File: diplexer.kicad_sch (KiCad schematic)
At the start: 27 parts, among them J1 Conn_Coaxial, J2 Conn_Coaxial, J3 Conn_Coaxial, J4 Conn_01x01_Pin, J5 Conn_01x01_Pin, J6 Conn_01x01_Pin, J7 Conn_01x01_Pin

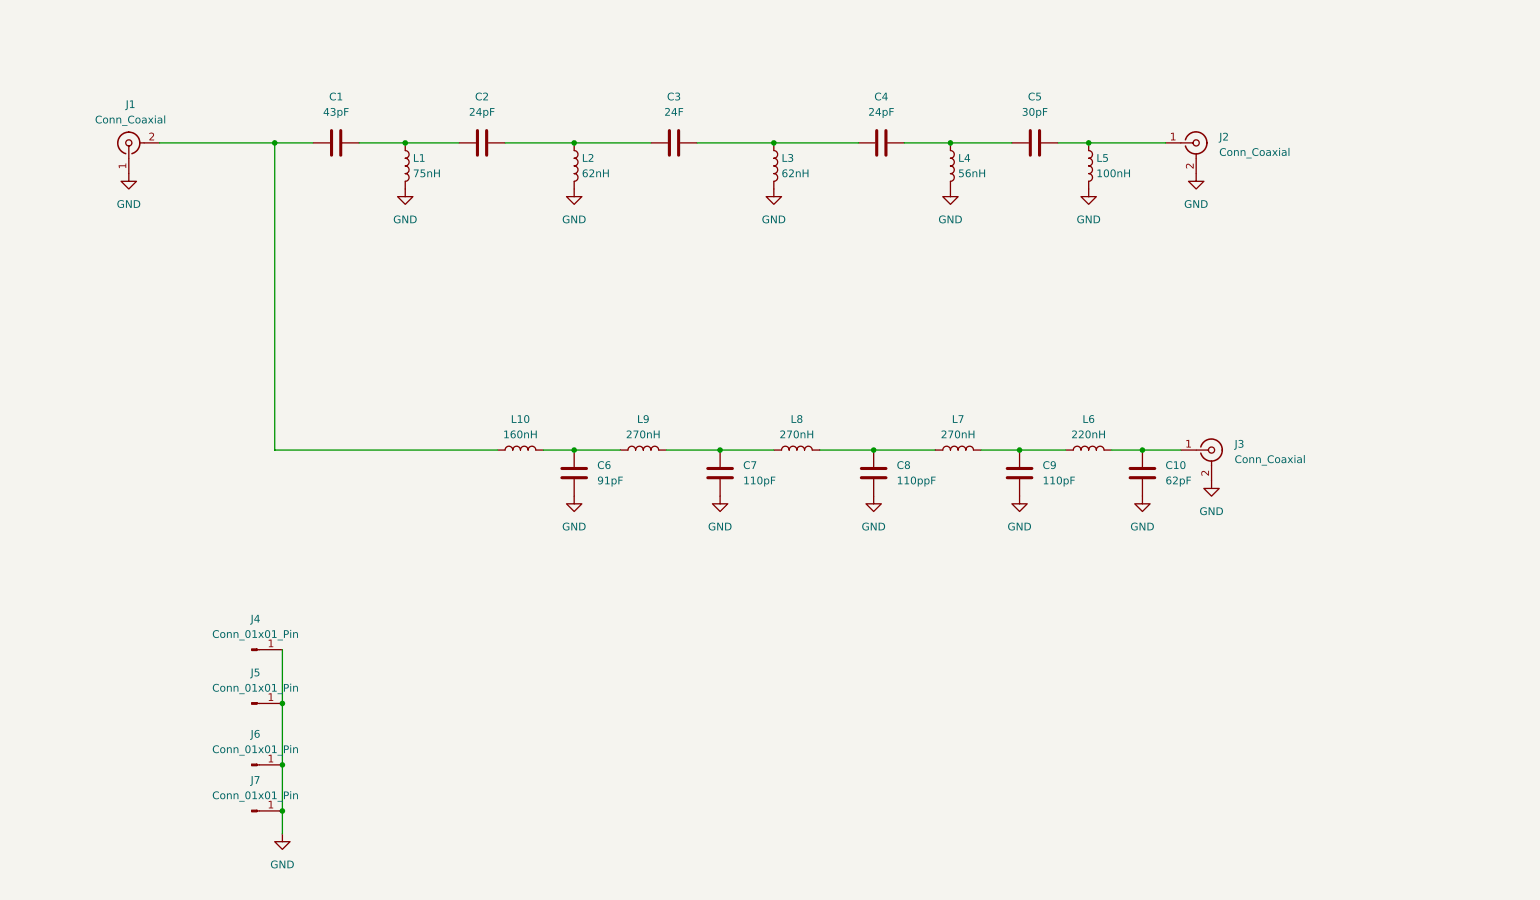
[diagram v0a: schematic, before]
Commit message: Add files via upload
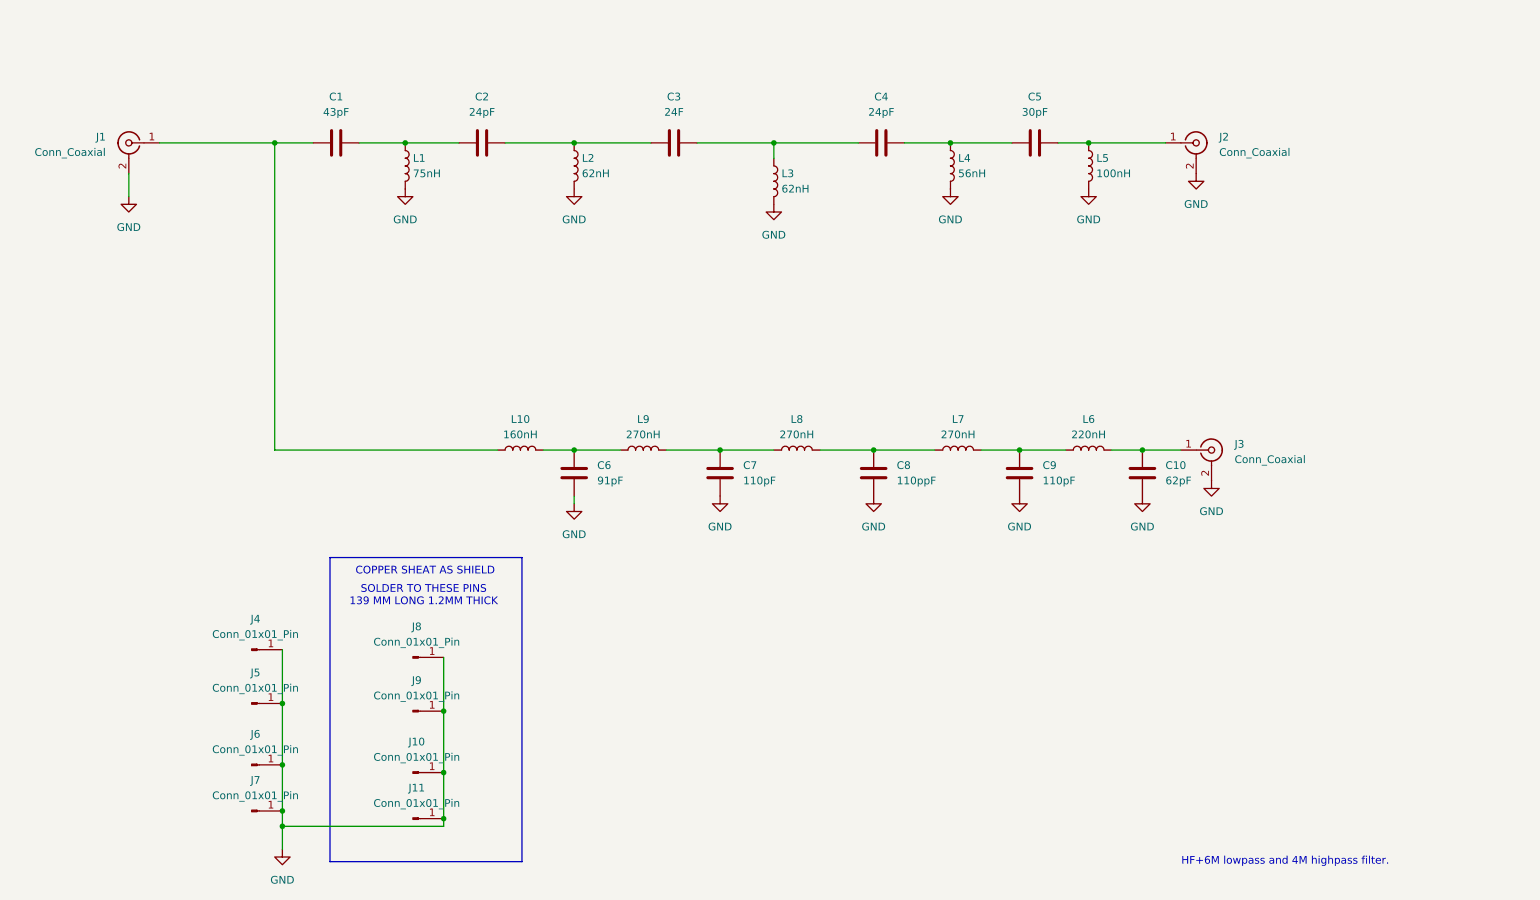
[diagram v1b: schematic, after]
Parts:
- added J10, J11, J8, J9: Conn_01x01_Pin, MountingHole:MountingHole_3.2mm_M3_DIN965_Pad, symbol Connector:Conn_01x01_Pin
- J4, J5, J6, J7: footprint MountingHole:MountingHole_3.2mm_M3 -> MountingHole:MountingHole_3.2mm_M3_DIN965_Pad
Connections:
- net GND: now also J1.2 (Ext), J10.1 (Pin_1), J11.1 (Pin_1), J8.1 (Pin_1), J9.1 (Pin_1); no longer J1.1 (In)
- net at C1.1, L10.1: now also J1.1 (In); no longer J1.2 (Ext)
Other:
- note added: "COPPER SHEAT AS SHIELD"
- note added: "HF+6M lowpass and 4M highpass filter."
- note added: "SOLDER TO THESE PINS 139 MM LONG 1.2MM THICK"
- moved on the sheet: J1, L3

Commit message: Add files via upload
Updated capacitors foot prints to 2525 (QEEV Series)
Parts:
- C1, C10, C2, C3, C4, C5, C6, C7, C8, C9: footprint Capacitor_SMD:C_2220_5750Metric -> sparkfun-electromech:2525
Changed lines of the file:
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@@
 			)
 		)
-		(property "Footprint" "Capacitor_SMD:C_2220_5750Metric"
+		(property "Footprint" "sparkfun-electromech:2525"
 			(at 105.7148 104.14 0)
 			(effects
@@
 			)
 		)
-		(property "Footprint" "Capacitor_SMD:C_2220_5750Metric"
+		(property "Footprint" "sparkfun-electromech:2525"
 			(at 186.69 52.3748 0)
 			(effects
@@
 			)
 		)
-		(property "Footprint" "Capacitor_SMD:C_2220_5750Metric"
+		(property "Footprint" "sparkfun-electromech:2525"
 			(at 161.29 52.3748 0)
 			(effects
@@
 			)
 		)
-		(property "Footprint" "Capacitor_SMD:C_2220_5750Metric"
+		(property "Footprint" "sparkfun-electromech:2525"
 			(at 179.3748 104.14 0)
 			(effects
@@
 			)
 		)
-		(property "Footprint" "Capacitor_SMD:C_2220_5750Metric"
+		(property "Footprint" "sparkfun-electromech:2525"
 			(at 95.25 52.3748 0)
 			(effects
@@
 			)
 		)
-		(property "Footprint" "Capacitor_SMD:C_2220_5750Metric"
+		(property "Footprint" "sparkfun-electromech:2525"
 			(at 199.6948 104.14 0)
 			(effects
@@
 			)
 		)
-		(property "Footprint" "Capacitor_SMD:C_2220_5750Metric"
+		(property "Footprint" "sparkfun-electromech:2525"
 			(at 129.8448 104.14 0)
 			(effects
@@
 			)
 		)
-		(property "Footprint" "Capacitor_SMD:C_2220_5750Metric"
+		(property "Footprint" "sparkfun-electromech:2525"
 			(at 71.12 52.3748 0)
 			(effects
@@
 			)
 		)
-		(property "Footprint" "Capacitor_SMD:C_2220_5750Metric"
+		(property "Footprint" "sparkfun-electromech:2525"
 			(at 155.2448 104.14 0)
 			(effects
@@
 			)
 		)
-		(property "Footprint" "Capacitor_SMD:C_2220_5750Metric"
+		(property "Footprint" "sparkfun-electromech:2525"
 			(at 127 52.3748 0)
 			(effects

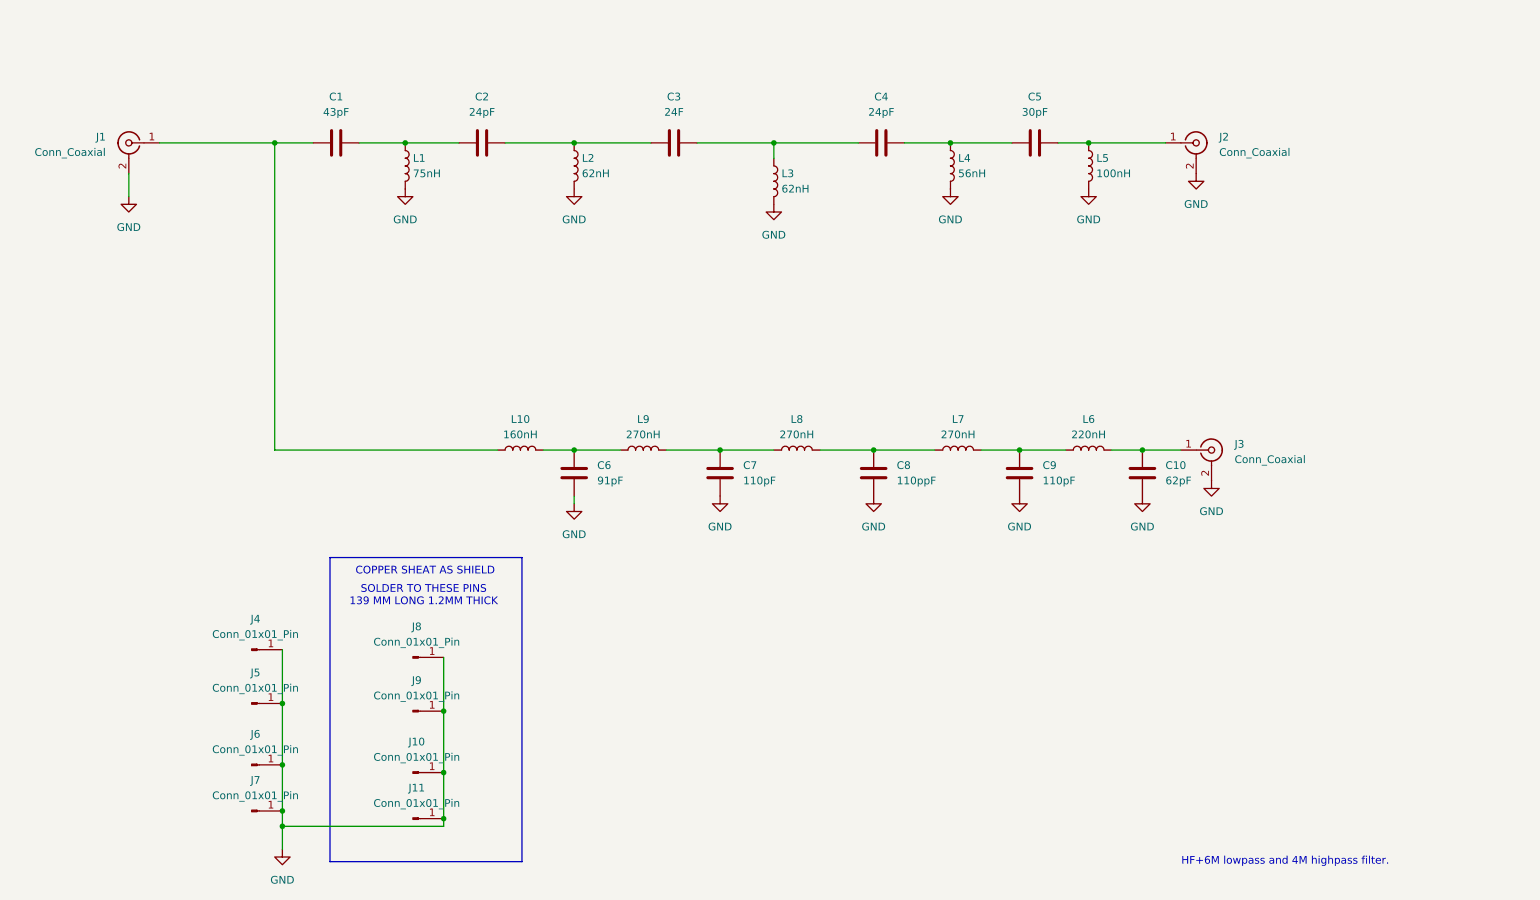
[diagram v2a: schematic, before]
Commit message: Add files via upload
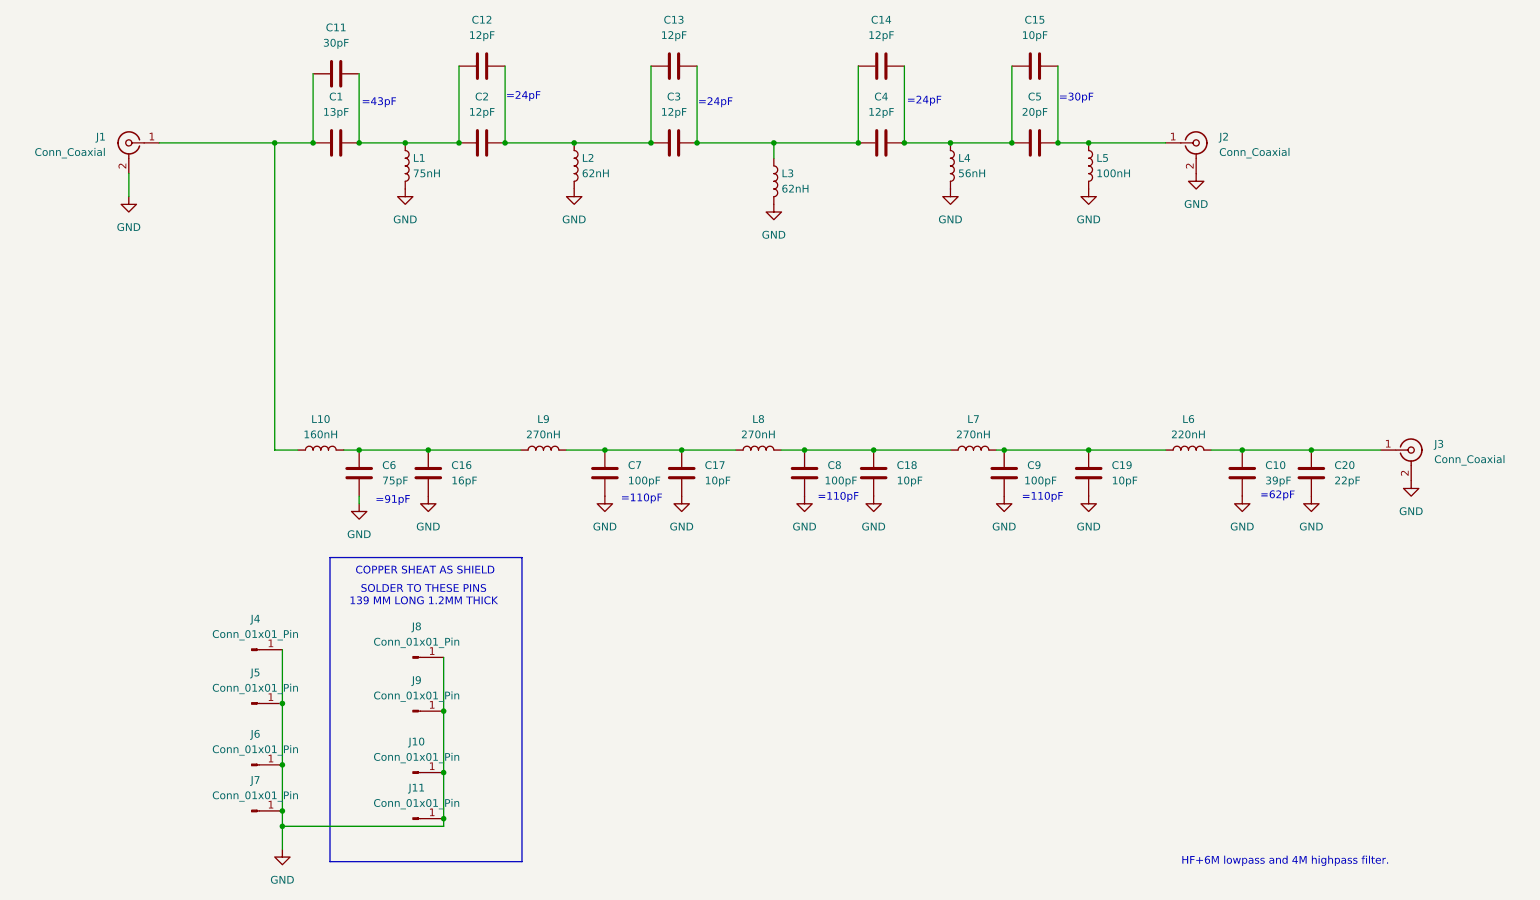
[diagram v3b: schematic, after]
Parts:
- added C11: 30pF, sparkfun-electromech:1111, symbol Device:C
- added C12, C13, C14: 12pF, sparkfun-electromech:1111, symbol Device:C
- added C15, C17, C18, C19: 10pF, sparkfun-electromech:1111, symbol Device:C
- added C16: 16pF, sparkfun-electromech:1111, symbol Device:C
- added C20: 22pF, sparkfun-electromech:1111, symbol Device:C
- C1: value 43pF -> 13pF; footprint sparkfun-electromech:2525 -> sparkfun-electromech:1111
- C10: value 62pF -> 39pF; footprint sparkfun-electromech:2525 -> sparkfun-electromech:1111
- C2, C4: value 24pF -> 12pF; footprint sparkfun-electromech:2525 -> sparkfun-electromech:1111
- C3: value 24F -> 12pF; footprint sparkfun-electromech:2525 -> sparkfun-electromech:1111
- C5: value 30pF -> 20pF; footprint sparkfun-electromech:2525 -> sparkfun-electromech:1111
- C6: value 91pF -> 75pF; footprint sparkfun-electromech:2525 -> sparkfun-electromech:1111
- C7, C9: value 110pF -> 100pF; footprint sparkfun-electromech:2525 -> sparkfun-electromech:1111
- C8: value 110ppF -> 100pF; footprint sparkfun-electromech:2525 -> sparkfun-electromech:1111
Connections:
- net GND: now also C16.2, C17.2, C18.2, C19.2, C20.2
- net at C6.2, L10.2, L9.1: now also C16.1
- net at C4.2, C5.1, L4.1: now also C14.2, C15.1
- net at C5.2, J2.1 (In), L5.1: now also C15.2
- net at C3.2, C4.1, L3.1: now also C13.2, C14.1
- net at C1.1, J1.1 (In), L10.1: now also C11.1
- net at C7.2, L8.1, L9.2: now also C17.1
- net at C8.2, L7.1, L8.2: now also C18.1
- net at C9.2, L6.1, L7.2: now also C19.1
- net at C1.2, C2.1, L1.1: now also C11.2, C12.1
- net at C2.2, C3.1, L2.1: now also C12.2, C13.1
- net at C10.2, J3.1 (In), L6.2: now also C20.1
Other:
- note added: "=110pF"
- note added: "=24pF"
- note added: "=30pF"
- note added: "=43pF"
- note added: "=62pF"
- note added: "=91pF"
- moved on the sheet: C10, C6, C7, C8, C9, J3, L10, L6, L7, L8, L9

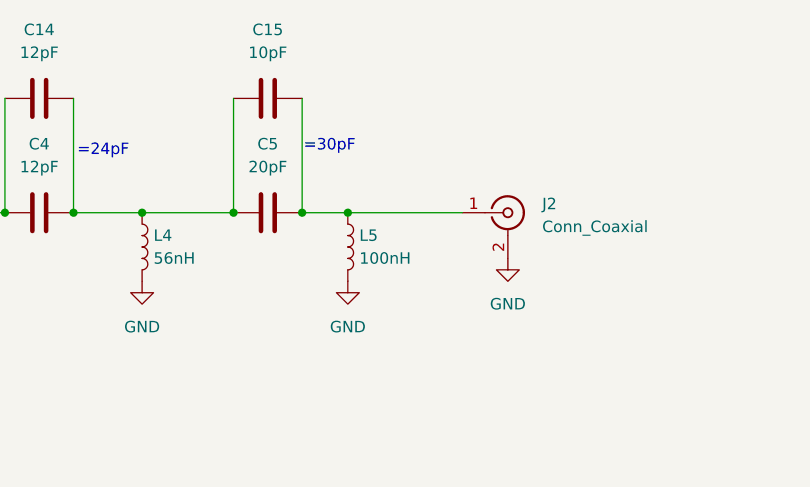
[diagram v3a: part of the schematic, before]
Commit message: Add files via upload
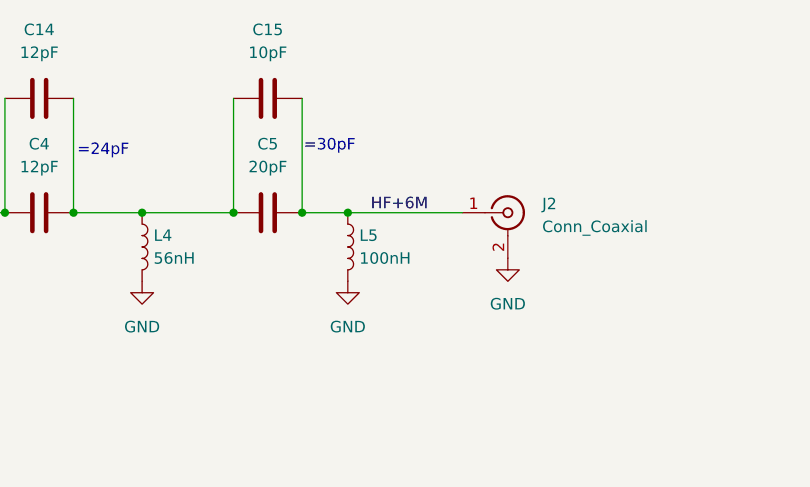
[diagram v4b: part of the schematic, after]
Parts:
- J2: footprint sparkfun-electromech:N-conn slanted -> sparkfun-electromech:UHF slanted
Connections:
- net HF+6M: now reaches C15.2, C5.2, J2.1 (In), L5.1
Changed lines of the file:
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@@
 		)
 	)
+	(label "HF+6M"
+		(at 194.31 53.34 0)
+		(fields_autoplaced yes)
+		(effects
+			(font
+				(size 1.27 1.27)
+			)
+			(justify left bottom)
+		)
+	)
 	(symbol
 		(lib_id "power:GND")
@@
 			)
 		)
-		(property "Footprint" "sparkfun-electromech:N-conn slanted"
+		(property "Footprint" "sparkfun-electromech:UHF slanted"
 			(at 209.296 44.45 0)
 			(effects

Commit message: Add files via upload
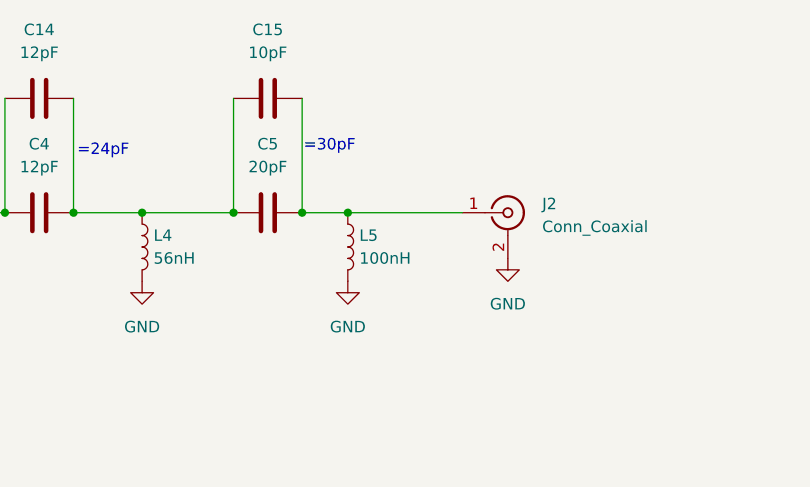
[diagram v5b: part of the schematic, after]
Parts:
- J2: footprint sparkfun-electromech:UHF slanted -> sparkfun-electromech:N-conn slanted
- J3: footprint sparkfun-electromech:N-conn slanted -> sparkfun-electromech:UHF slanted
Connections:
- net HF+6M: no longer names the net of C15.2, C5.2, J2.1 (In), L5.1
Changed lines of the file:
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@@
 		)
 	)
-	(label "HF+6M"
-		(at 194.31 53.34 0)
-		(fields_autoplaced yes)
-		(effects
-			(font
-				(size 1.27 1.27)
-			)
-			(justify left bottom)
-		)
-	)
 	(symbol
 		(lib_id "power:GND")
@@
 			)
 		)
-		(property "Footprint" "sparkfun-electromech:N-conn slanted"
+		(property "Footprint" "sparkfun-electromech:UHF slanted"
 			(at 245.11 104.14 0)
 			(effects
@@
 			)
 		)
-		(property "Footprint" "sparkfun-electromech:UHF slanted"
+		(property "Footprint" "sparkfun-electromech:N-conn slanted"
 			(at 209.296 44.45 0)
 			(effects
